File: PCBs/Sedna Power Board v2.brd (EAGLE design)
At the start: 50 x 32 mm, 21 parts

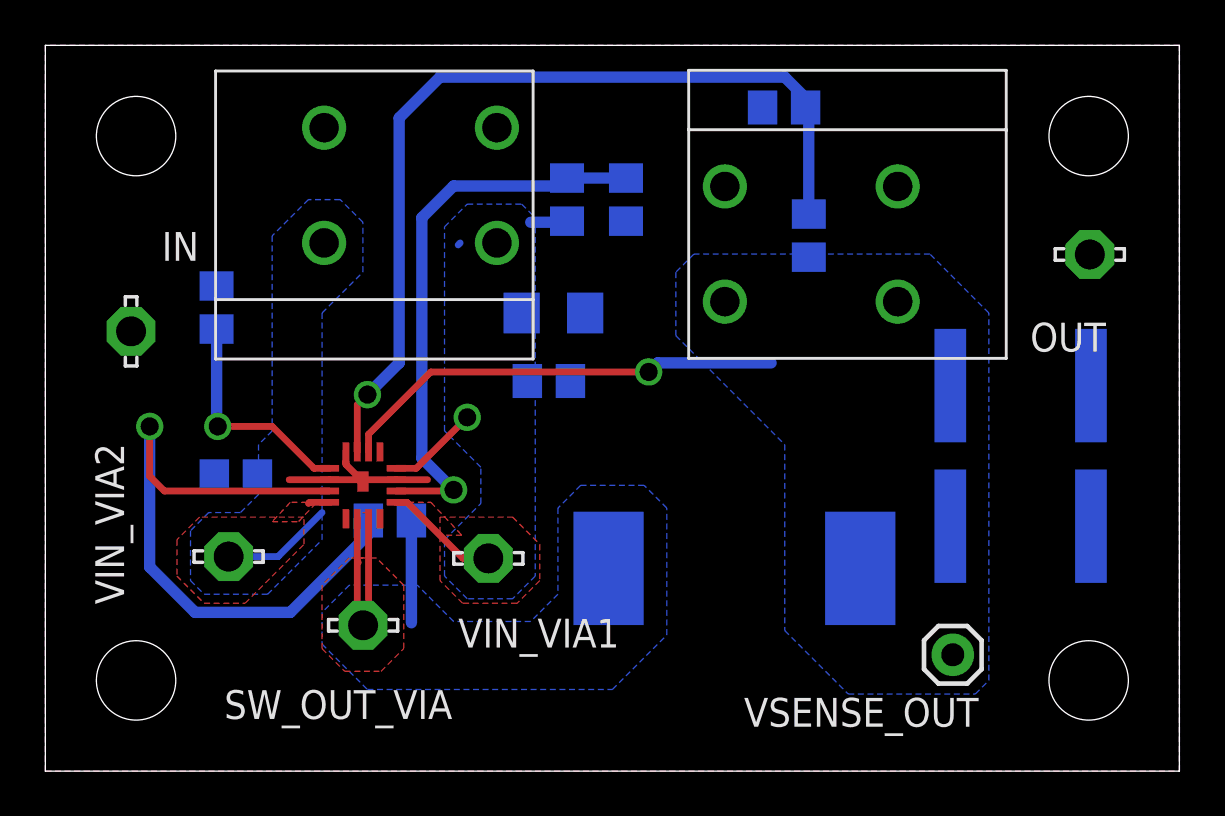
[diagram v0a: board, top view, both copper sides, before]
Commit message: v2.0.2 of the power board - still prototyping, still learning...
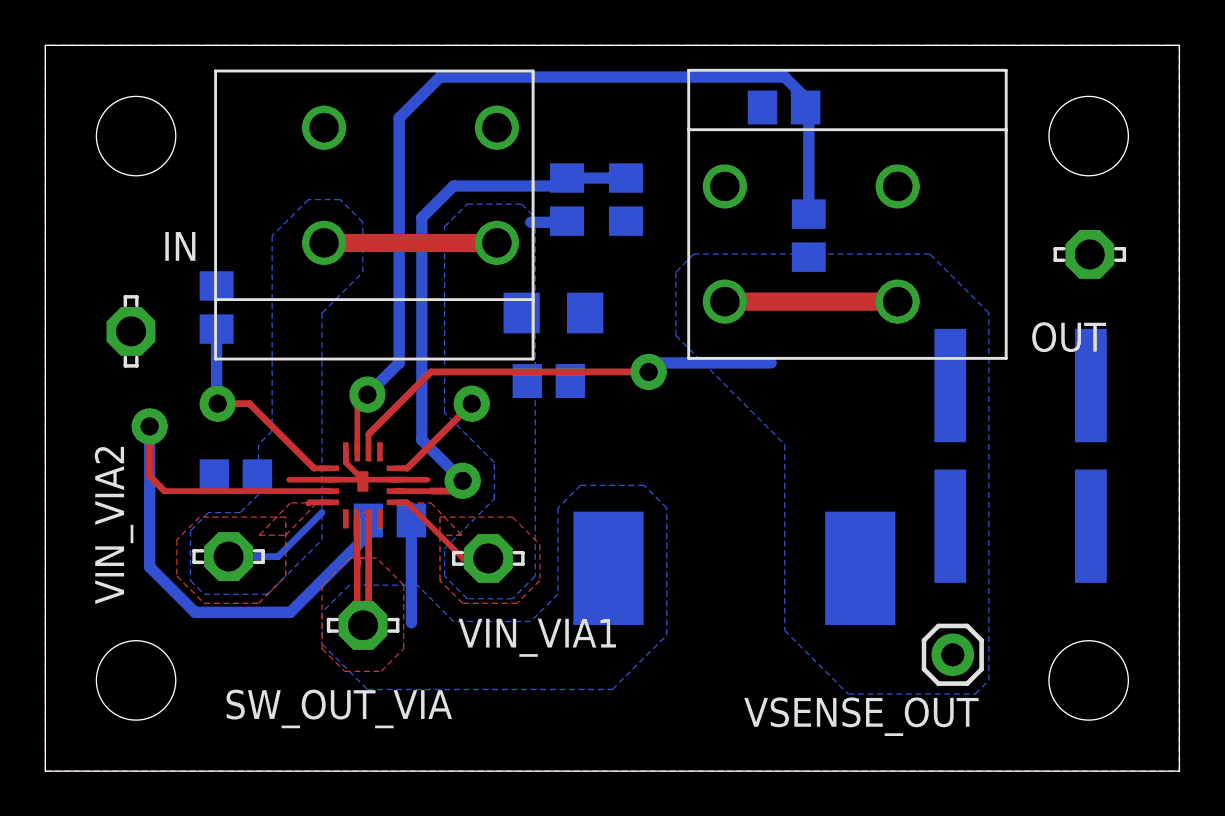
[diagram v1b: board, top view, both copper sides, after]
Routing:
- net V_IN: track 16.8 -> 24.8 mm
- net V_OUT: track 19.8 -> 27.4 mm
- net VCC: track 10.0 -> 9.42 mm
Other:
- board text added: "Sedna Power Board v2.0.2"
- board text removed: "Sedna Power Board v2.0"
